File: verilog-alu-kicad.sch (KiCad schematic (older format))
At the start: 9 parts

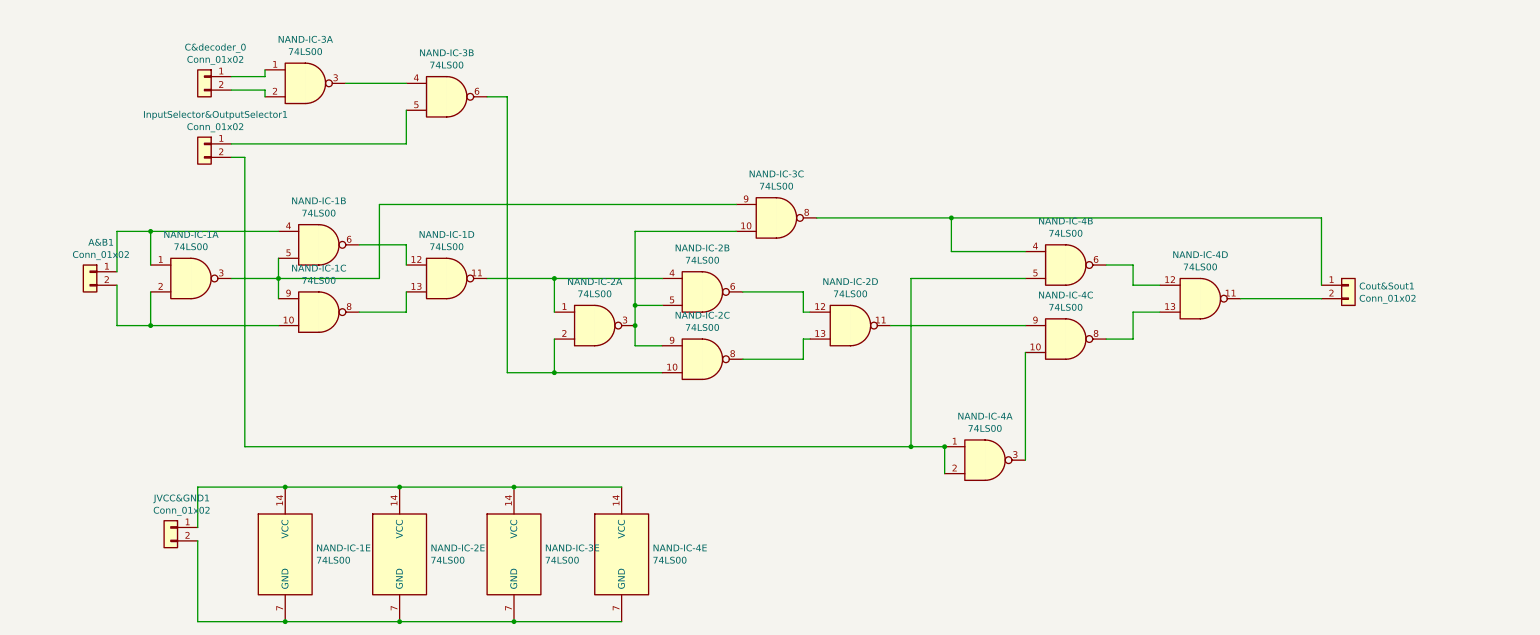
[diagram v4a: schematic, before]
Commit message: 完成したんじゃね？
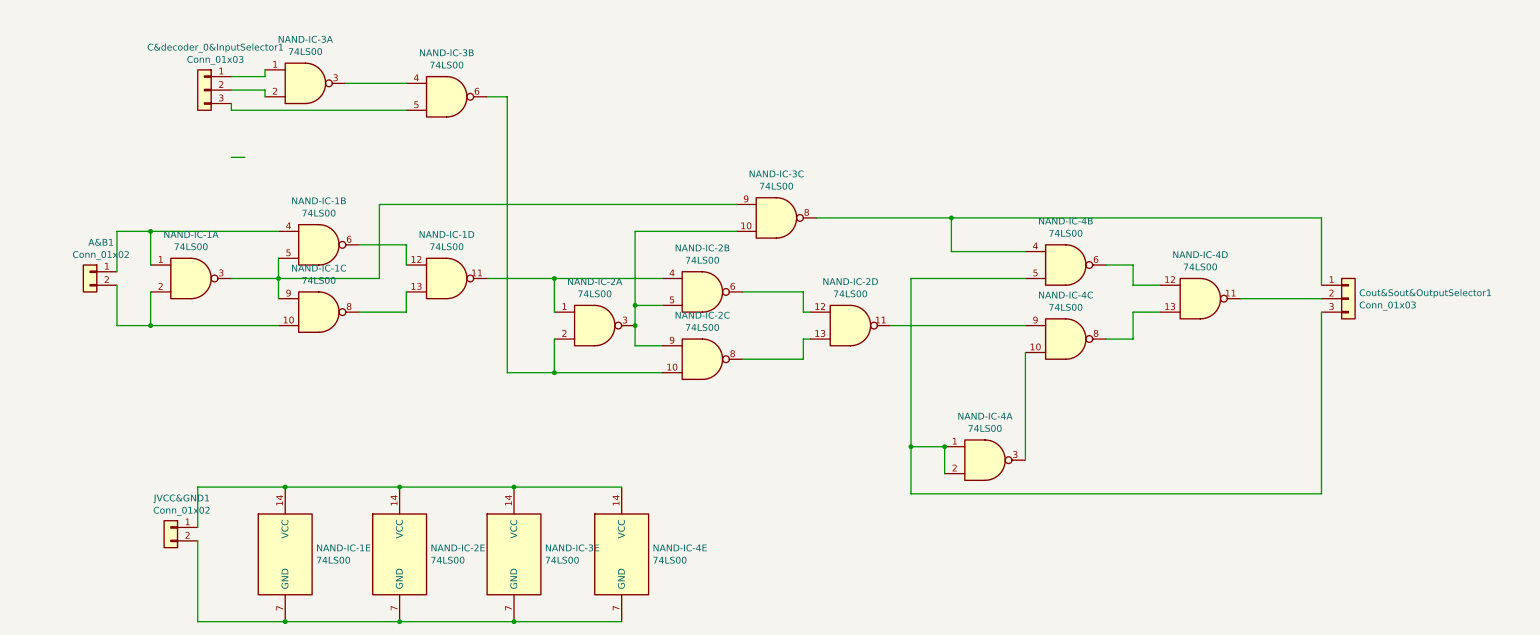
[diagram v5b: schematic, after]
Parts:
- removed C&decoder_0, Cout&Sout1, InputSelector&OutputSelector1: Conn_01x02, Connector_PinHeader_2.54mm:PinHeader_1x02_P2.54mm_Vertical, symbol Connector_Generic:Conn_01x02
- added C&decoder_0&InputSelector1, Cout&Sout&OutputSelector1: Conn_01x03, Connector_PinHeader_2.54mm:PinHeader_1x03_P2.54mm_Horizontal, symbol Connector_Generic:Conn_01x03
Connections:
- net at NAND-IC-3.1: now also C&decoder_0&InputSelector1.1 (Pin_1)
- net at NAND-IC-3.2: now also C&decoder_0&InputSelector1.2 (Pin_2)
- net at NAND-IC-3.5: now also C&decoder_0&InputSelector1.3 (Pin_3)
- net at NAND-IC-3.8, NAND-IC-4.4: now also Cout&Sout&OutputSelector1.1 (Pin_1)
- net at NAND-IC-4.1, NAND-IC-4.2, NAND-IC-4.5: now also Cout&Sout&OutputSelector1.3 (Pin_3)
- net at NAND-IC-4.11: now also Cout&Sout&OutputSelector1.2 (Pin_2)
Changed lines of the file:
@@
 	2350 1150 2350 1200
-Wire Wire Line
-	2100 1550 3400 1550
-Wire Wire Line
-	3400 1300 3400 1550
 Wire Wire Line
 	2100 2550 2450 2550
@@
 Wire Wire Line
 	2100 1650 2200 1650
-Wire Wire Line
-	2200 3800 7150 3800
-Wire Wire Line
-	2200 1650 2200 3800
 Wire Wire Line
 	7450 2100 10200 2100
@@
 $EndComp
 $Comp
-L Connector_Generic:Conn_01x02 InputSelector&OutputSelector1
-U 1 1 5E0DD4AF
-P 1900 1550
-F 0 "InputSelector&OutputSelector1" H 1818 1767 50  0000 C CNN
-F 1 "Conn_01x02" H 1818 1676 50  0000 C CNN
-F 2 "Connector_PinHeader_2.54mm:PinHeader_1x02_P2.54mm_Vertical" H 1900 1550 50  0001 C CNN
-F 3 "~" H 1900 1550 50  0001 C CNN
-	1    1900 1550
+L Connector_Generic:Conn_01x03 C&decoder_0&InputSelector1
+U 1 1 5E130E52
+P 1900 1150
+F 0 "C&decoder_0&InputSelector1" H 1818 1467 50  0000 C CNN
+F 1 "Conn_01x03" H 1818 1376 50  0000 C CNN
+F 2 "Connector_PinHeader_2.54mm:PinHeader_1x03_P2.54mm_Horizontal" H 1900 1150 50  0001 C CNN
+F 3 "~" H 1900 1150 50  0001 C CNN
+	1    1900 1150
 	-1   0    0    -1
 $EndComp
+Wire Wire Line
+	3400 1300 2100 1300
+Wire Wire Line
+	2100 1300 2100 1250
 $Comp
-L Connector_Generic:Conn_01x02 C&decoder_0
-U 1 1 5E0E8985
-P 1900 1050
-F 0 "C&decoder_0" H 1818 1267 50  0000 C CNN
-F 1 "Conn_01x02" H 1818 1176 50  0000 C CNN
-F 2 "Connector_PinHeader_2.54mm:PinHeader_1x02_P2.54mm_Vertical" H 1900 1050 50  0001 C CNN
-F 3 "~" H 1900 1050 50  0001 C CNN
-	1    1900 1050
-	-1   0    0    -1
-$EndComp
-$Comp
-L Connector_Generic:Conn_01x02 Cout&Sout1
-U 1 1 5E1AD419
-P 10400 2600
-F 0 "Cout&Sout1" H 10480 2592 50  0000 L CNN
-F 1 "Conn_01x02" H 10480 2501 50  0000 L CNN
-F 2 "Connector_PinHeader_2.54mm:PinHeader_1x02_P2.54mm_Vertical" H 10400 2600 50  0001 C CNN
-F 3 "~" H 10400 2600 50  0001 C CNN
-	1    10400 2600
+L Connector_Generic:Conn_01x03 Cout&Sout&OutputSelector1
+U 1 1 5E1DEB25
+P 10400 2700
+F 0 "Cout&Sout&OutputSelector1" H 10480 2742 50  0000 L CNN
+F 1 "Conn_01x03" H 10480 2651 50  0000 L CNN
+F 2 "Connector_PinHeader_2.54mm:PinHeader_1x03_P2.54mm_Horizontal" H 10400 2700 50  0001 C CNN
+F 3 "~" H 10400 2700 50  0001 C CNN
+	1    10400 2700
 	1    0    0    -1
 $EndComp
+Wire Wire Line
+	7150 3800 7150 4150
+Wire Wire Line
+	7150 4150 10200 4150
+Wire Wire Line
+	10200 4150 10200 2800
 $EndSCHEMATC
